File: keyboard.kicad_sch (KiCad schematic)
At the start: 73 parts, among them J1 Conn01_02, J2 Conn_01x04_Pin, J3 USB_C_Receptacle_USB2.0_16P, J4 Conn_01x06_Socket, Q1 Q_PMOS_SGD, SW1 SW_Push, SW10 SW_Push, SW11 SW_Push, SW12 SW_Push, SW13 SW_Push, SW14 SW_Push, SW15 SW_Push, SW16 SW_Push, SW17 SW_Push, SW18 SW_Push, SW19 SW_Push, SW2 SW_Push, SW20 SW_Push, SW21 SW_Push, SW22 SW_Push, SW23 SW_Push, SW3 SW_Push, SW4 SW_Push, SW5 SW_Push, SW6 SW_Push, SW7 SW_Push, SW8 SW_Push, SW9 SW_Push, U1 MDBT50Q-1MV2, U2 MCP73831-2-OT, U3 IS31FL3733-TQ

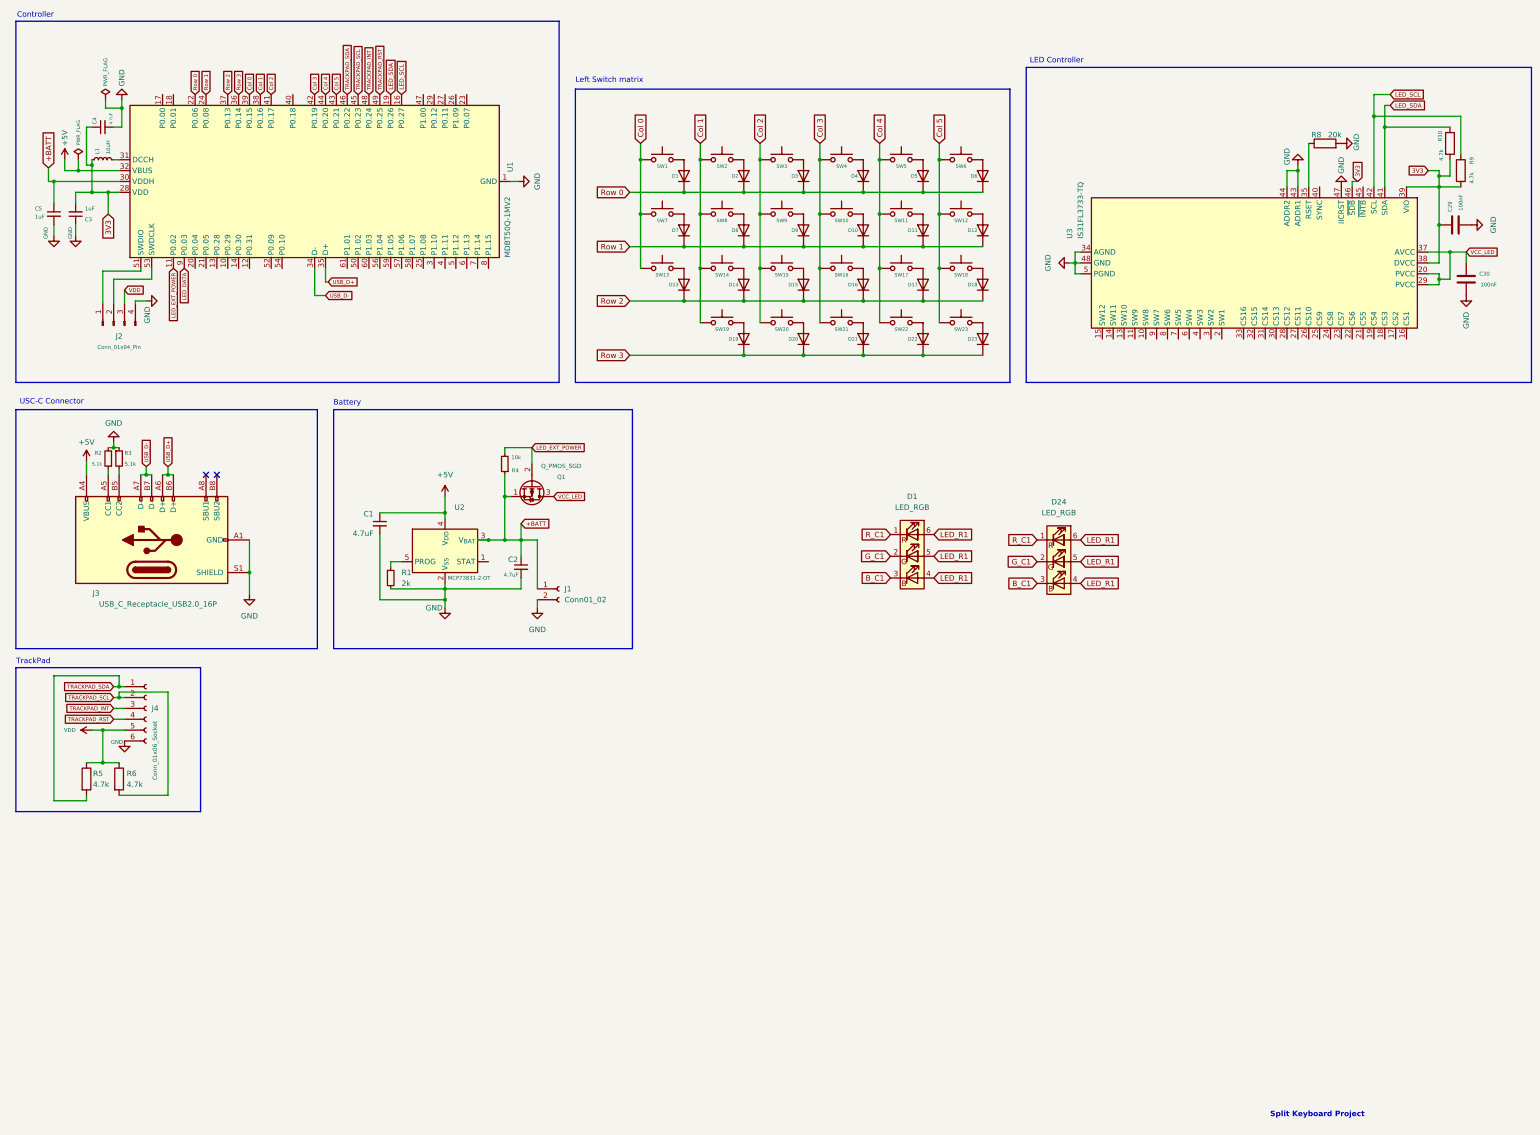
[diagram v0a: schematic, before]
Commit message: new updates
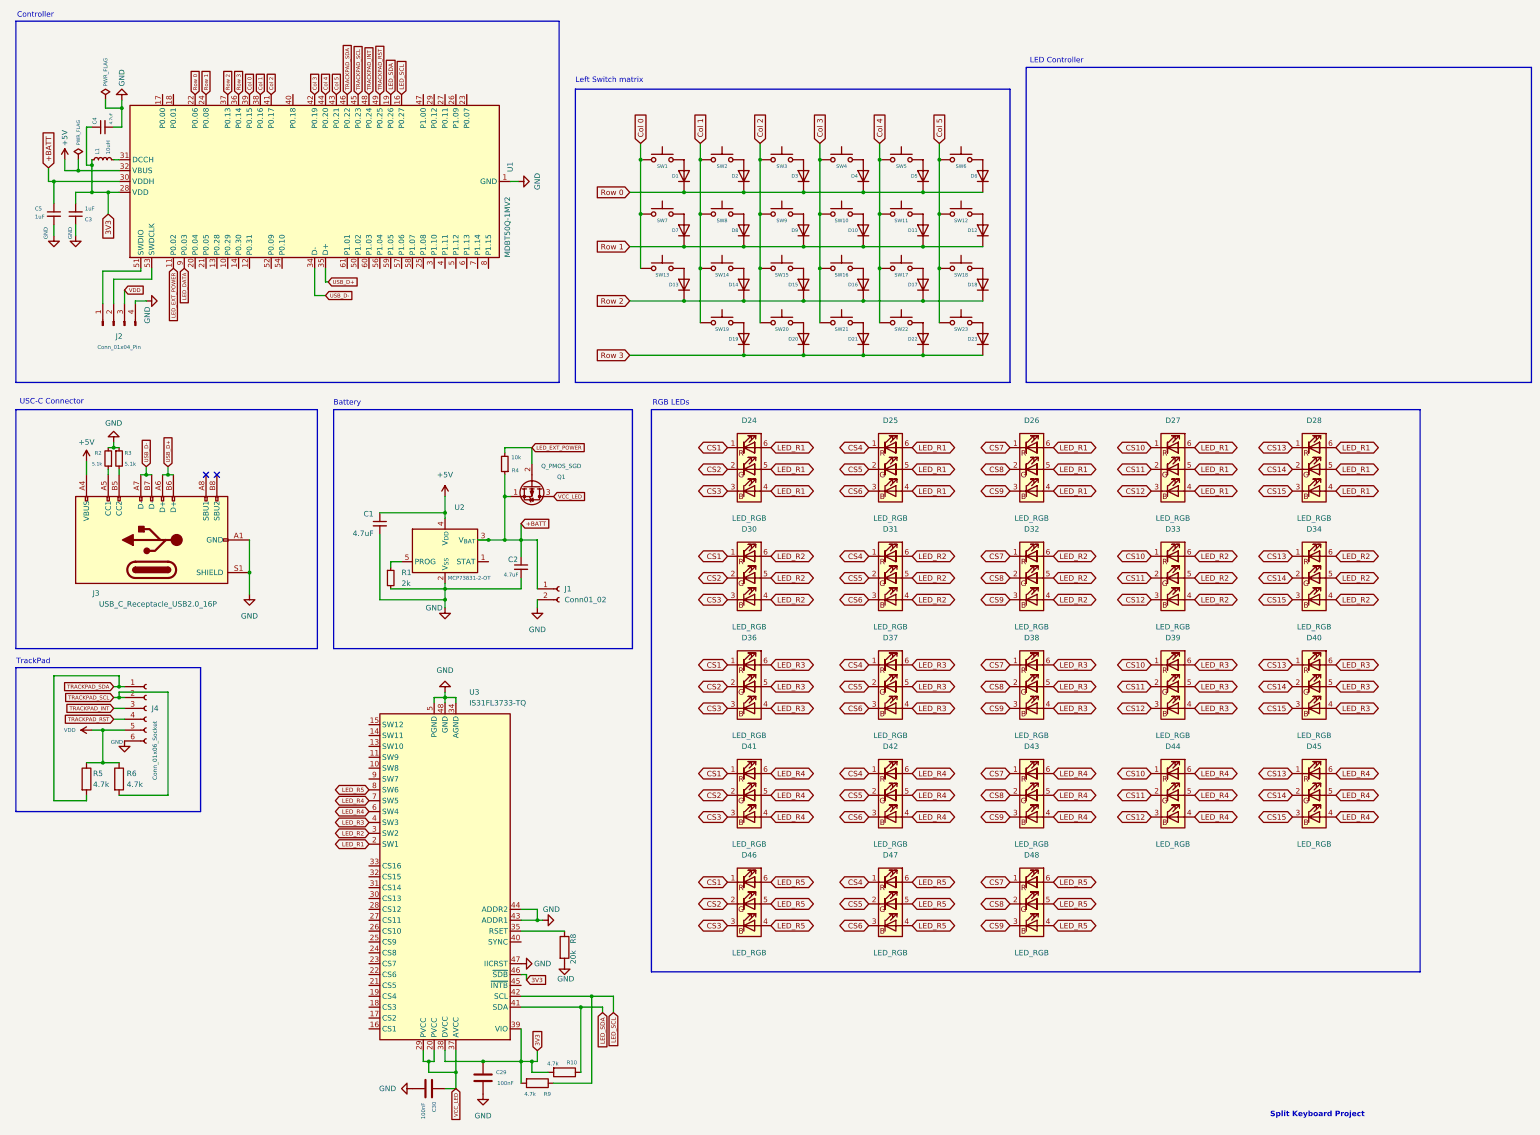
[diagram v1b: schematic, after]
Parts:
- removed D1: LED_RGB, symbol Device:LED_RGB
- added D25, D26, D27, D28, D30, D31, D32, D33, D34, D36, D37, D38, D39, D40, D41, D42, D43, D44, D45, D46, D47, D48: LED_RGB, symbol Device:LED_RGB
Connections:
- net LED_R1: now also U3.2 (SW1), D25.4 (BA), D25.5 (GA), D25.6 (RA), D26.4 (BA), D26.5 (GA), D26.6 (RA), D27.4 (BA), D27.5 (GA), D27.6 (RA), D28.4 (BA), D28.5 (GA), D28.6 (RA)
- net LED_R2: now reaches U3.3 (SW2)
- net LED_R2: now also D30.4 (BA), D30.5 (GA), D30.6 (RA), D31.4 (BA), D31.5 (GA), D31.6 (RA), D32.4 (BA), D32.5 (GA), D32.6 (RA), D33.4 (BA), D33.5 (GA), D33.6 (RA), D34.4 (BA), D34.5 (GA), D34.6 (RA)
- net LED_R3: now reaches U3.4 (SW3)
- net LED_R3: now also D36.4 (BA), D36.5 (GA), D36.6 (RA), D37.4 (BA), D37.5 (GA), D37.6 (RA), D38.4 (BA), D38.5 (GA), D38.6 (RA), D39.4 (BA), D39.5 (GA), D39.6 (RA), D40.4 (BA), D40.5 (GA), D40.6 (RA)
- net LED_R4: now reaches U3.6 (SW4)
- net LED_R4: now also U3.7 (SW5), D41.4 (BA), D41.5 (GA), D41.6 (RA), D42.4 (BA), D42.5 (GA), D42.6 (RA), D43.4 (BA), D43.5 (GA), D43.6 (RA), D44.4 (BA), D44.5 (GA), D44.6 (RA), D45.4 (BA), D45.5 (GA), D45.6 (RA)
- net LED_R5: now reaches U3.8 (SW6)
- net LED_R5: now also D46.4 (BA), D46.5 (GA), D46.6 (RA), D47.4 (BA), D47.5 (GA), D47.6 (RA), D48.4 (BA), D48.5 (GA), D48.6 (RA)
- net B_C1 renamed CS3
- net CS3: now also D30.3 (BK), D36.3 (BK), D41.3 (BK), D46.3 (BK)
- net G_C1 renamed CS2
- net CS2: now also D30.2 (GK), D36.2 (GK), D41.2 (GK), D46.2 (GK)
- net R_C1 renamed CS1
- net CS1: now also D30.1 (RK), D36.1 (RK), D41.1 (RK), D46.1 (RK)
- new net CS10: D27.1 (RK), D33.1 (RK), D39.1 (RK), D44.1 (RK)
- new net CS11: D27.2 (GK), D33.2 (GK), D39.2 (GK), D44.2 (GK)
- new net CS12: D27.3 (BK), D33.3 (BK), D39.3 (BK), D44.3 (BK)
- new net CS13: D28.1 (RK), D34.1 (RK), D40.1 (RK), D45.1 (RK)
- new net CS14: D28.2 (GK), D34.2 (GK), D40.2 (GK), D45.2 (GK)
- new net CS15: D28.3 (BK), D34.3 (BK), D40.3 (BK), D45.3 (BK)
- new net CS4: D25.1 (RK), D31.1 (RK), D37.1 (RK), D42.1 (RK), D47.1 (RK)
- new net CS5: D25.2 (GK), D31.2 (GK), D37.2 (GK), D42.2 (GK), D47.2 (GK)
- new net CS6: D25.3 (BK), D31.3 (BK), D37.3 (BK), D42.3 (BK), D47.3 (BK)
- new net CS7: D26.1 (RK), D32.1 (RK), D38.1 (RK), D43.1 (RK), D48.1 (RK)
- new net CS8: D26.2 (GK), D32.2 (GK), D38.2 (GK), D43.2 (GK), D48.2 (GK)
- new net CS9: D26.3 (BK), D32.3 (BK), D38.3 (BK), D43.3 (BK), D48.3 (BK)
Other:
- note added: "RGB LEDs"
- moved on the sheet: C29, C30, R10, R8, R9, U3
